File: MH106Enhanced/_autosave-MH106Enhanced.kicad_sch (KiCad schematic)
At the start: 44 parts, among them J1 Pin 1-20, J2 Pin 21 - 40, J3 5-15V, J4 USB Pins, J5 Debug, J6 I2C, Q1 BSS138, Q2 BSS138, U1 RP2040, U2 TPIC6C595D, U3 TPIC6C595D, U4 TPIC6C595D, U5 AMS1117-3.3, U6 W25Q128JVS, U7 ASDMB-xxxMHz

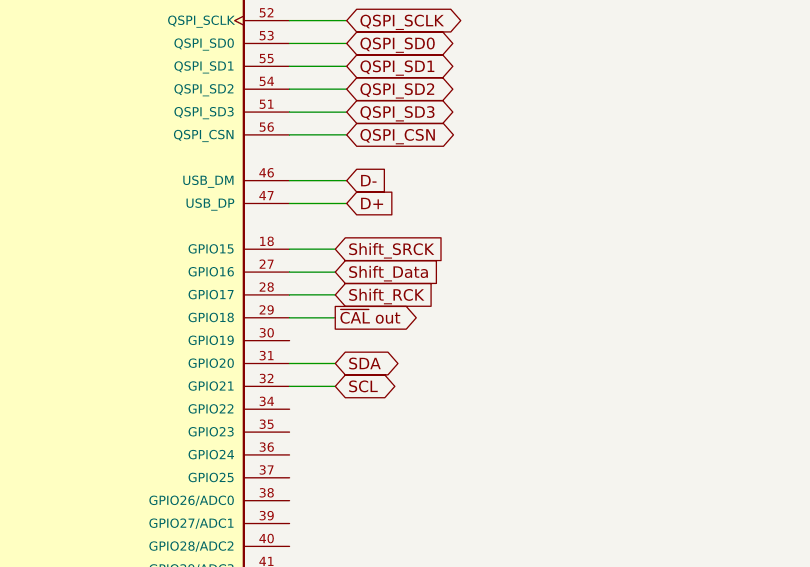
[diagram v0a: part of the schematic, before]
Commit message: Nearly DONE
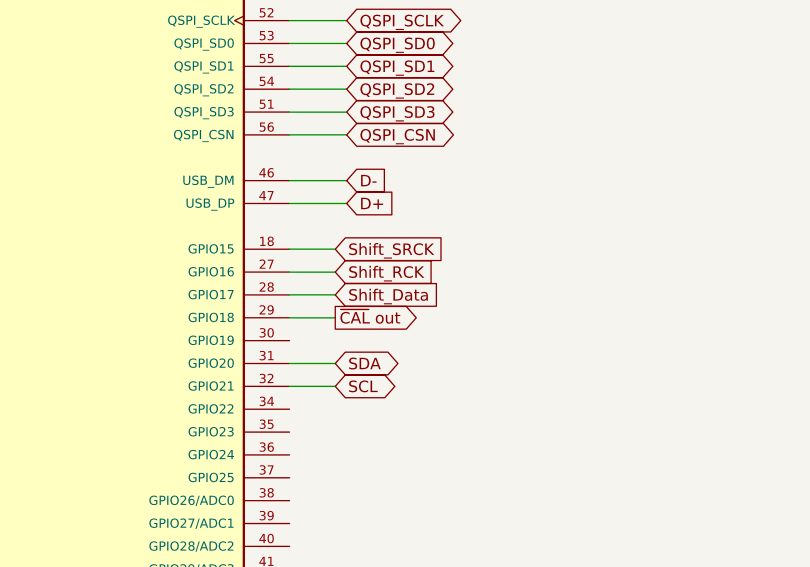
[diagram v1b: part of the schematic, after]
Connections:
- net Shift_Data: now also U1.28 (GPIO17); no longer U1.27 (GPIO16)
- net Shift_RCK: now also U1.27 (GPIO16); no longer U1.28 (GPIO17)
